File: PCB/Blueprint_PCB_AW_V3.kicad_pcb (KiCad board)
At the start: 2 copper layers, 100 x 100 mm, 37 parts, among them J2 Conn_01x04_Pin, SW1 SW_Push, SW10 SW_Push, SW11 SW_Push, SW12 SW_Push, SW13 SW_Push, SW14 SW_Push, SW15 SW_Push, SW16 SW_Push, SW17 RotaryEncoder_Switch, SW2 SW_Push, SW3 SW_Push, SW4 SW_Push, SW5 SW_Push, SW6 SW_Push, SW7 SW_Push, SW8 SW_Push, SW9 SW_Push, U1 XIAO-RP2040-DIP

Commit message: changes
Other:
- board text added: "Designed in Mürztal by wetzi"
- board text removed: "Made in Mürztal by wetzi"
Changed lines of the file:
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@@
 			(outputformat 1)
 			(mirror no)
-			(drillshape 1)
+			(drillshape 0)
 			(scaleselection 1)
-			(outputdirectory "")
+			(outputdirectory "../Production/gebers")
 		)
 	)
@@
 		)
 	)
-	(gr_text "Made in Mürztal\nby wetzi"
+	(gr_text "Designed in Mürztal\nby wetzi"
 		(at 93.5355 112.522 0)
 		(layer "Edge.Cuts")

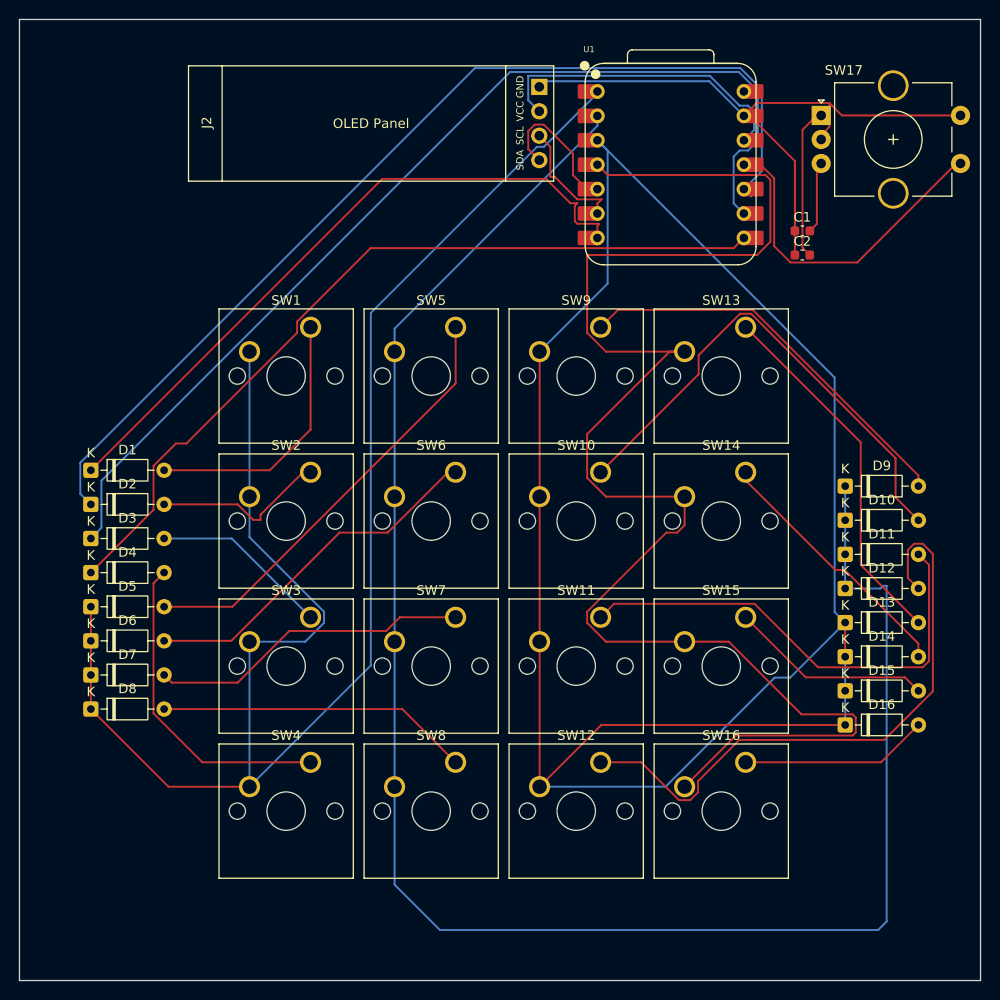
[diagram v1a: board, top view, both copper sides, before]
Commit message: big changes I lowkey designed new board
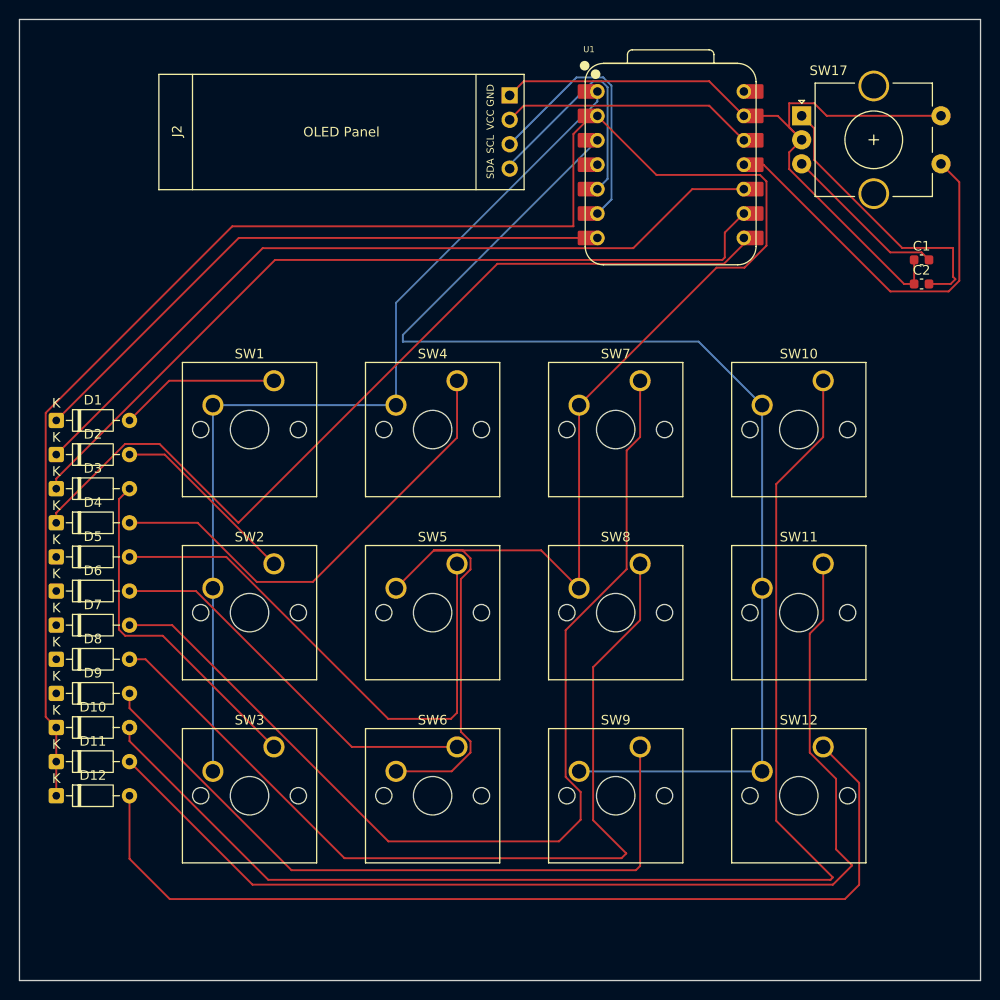
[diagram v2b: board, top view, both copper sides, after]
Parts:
- removed D13, D14, D15, D16: D, Diode_THT:D_DO-35_SOD27_P7.62mm_Horizontal
- removed SW13, SW14, SW15, SW16: SW_Push, Button_Switch_Keyboard:SW_Cherry_MX_1.00u_PCB
- moved D10 84.9 mm to (94.2, 88.2)
- moved D11 84.9 mm to (94.2, 91.7)
- moved D12 84.9 mm to (94.2, 95.2)
- moved D9 84.9 mm to (94.2, 84.6)
- moved SW9 43.9 mm to (154.9, 90.2)
- moved SW4 42.5 mm to (135.9, 52.1)
- moved SW7 31.2 mm to (154.9, 52.1)
- moved SW6 28.6 mm to (135.9, 90.2)
- moved SW8 28.2 mm to (154.9, 71.1)
- moved SW10 25.0 mm to (174.0, 52.1)
- moved SW5 24.6 mm to (135.9, 71.1)
- moved SW11 23.8 mm to (174.0, 71.1)
- moved SW12 23.2 mm to (174.0, 90.2)
- moved SW3 14.0 mm to (116.8, 90.2)
- moved C1 12.8 mm to (184.2, 39.5)
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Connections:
- U1 pad 4: COL4 -> unconnected-(U1-GPIO29/ADC3/A3-Pad4)
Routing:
- net COL4: track 164.7 -> 0.00 mm
- net COL3: track 215.5 -> 126.6 mm
- net Net-(D10-A): track 52.4 -> 136.8 mm
- net COL1: track 173.3 -> 98.5 mm
- net Net-(D7-A): track 33.5 -> 106.7 mm
- net Net-(D11-A): track 49.3 -> 115.1 mm
- net Net-(D8-A): track 32.6 -> 94.1 mm
- net COL2: track 192.3 -> 244.7 mm
- net Net-(D13-A): track 38.2 -> 0.00 mm
- net Net-(D12-A): track 63.6 -> 100.7 mm
- net Net-(D9-A): track 42.1 -> 74.2 mm
- net Net-(D14-A): track 27.2 -> 0.00 mm
- net ROW2: track 105.8 -> 83.0 mm
- net ROW3: track 108.0 -> 85.5 mm
- net Net-(D15-A): track 21.1 -> 0.00 mm
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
